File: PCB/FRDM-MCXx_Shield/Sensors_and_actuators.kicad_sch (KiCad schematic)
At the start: 15 parts, among them M1 Motor_Servo, U2 M95010-RMN6TP, U3 LM35-D

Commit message: Fixed labeling
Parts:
- U2: footprint SOIC127P600X175-8N -> SamacSys:SOIC127P600X175-8N
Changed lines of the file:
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@@
 			)
 		)
-		(property "Footprint" "SOIC127P600X175-8N"
+		(property "Footprint" "SamacSys:SOIC127P600X175-8N"
 			(at 251.46 213.03 0)
 			(effects

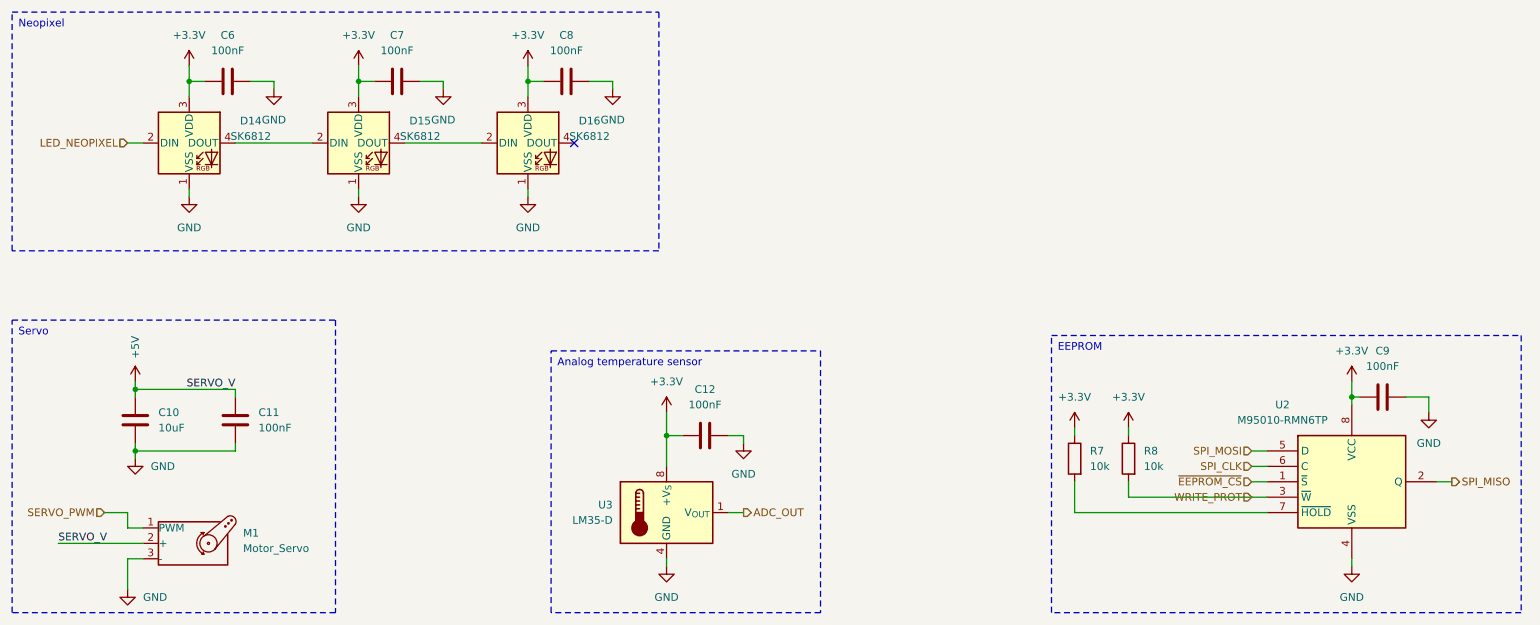
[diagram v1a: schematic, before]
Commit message: Updated PCB
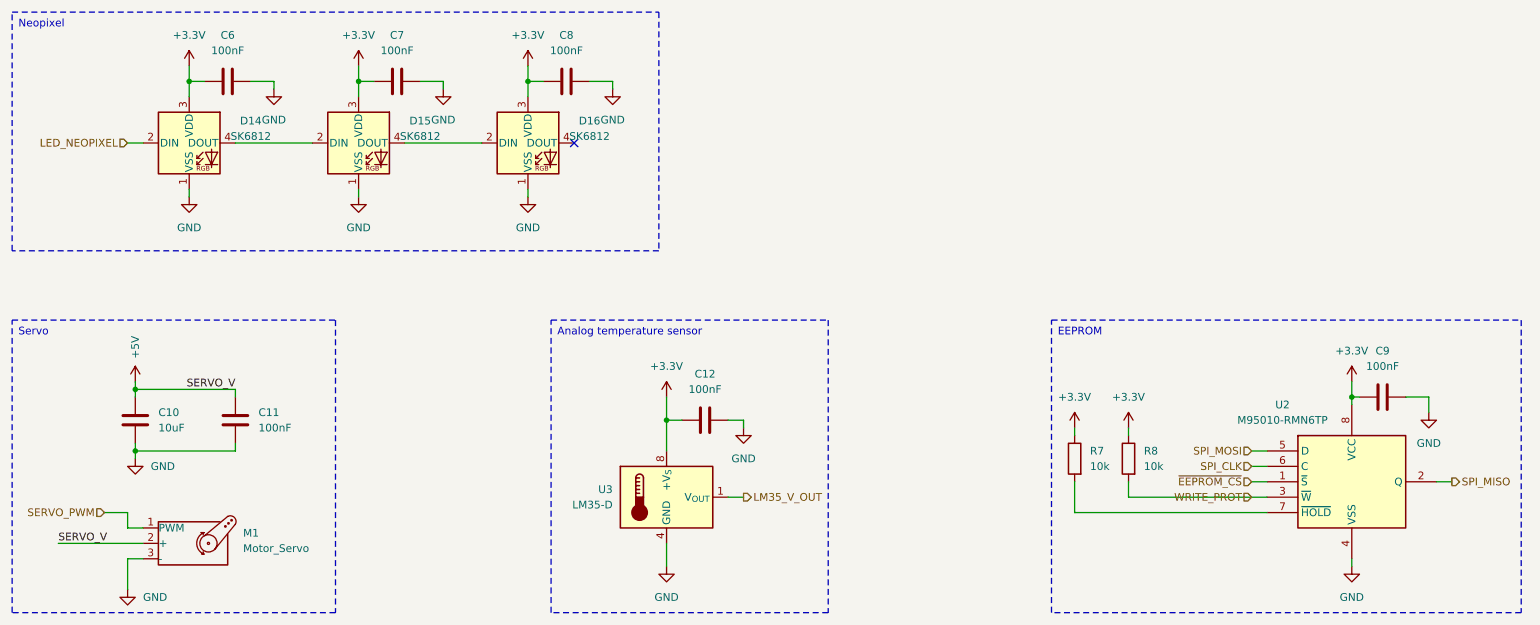
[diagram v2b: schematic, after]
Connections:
- net ADC_OUT renamed LM35_V_OUT
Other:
- moved on the sheet: C12, U3
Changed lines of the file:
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@@
 	(title_block
 		(title "Sensors & actuators")
-		(date "2024-04-26")
+		(date "2024-05-05")
 		(rev "V2.0")
 		(company "HAN")
@@
 	)
 	(junction
-		(at 128.27 113.03)
+		(at 128.27 110.49)
 		(diameter 0)
 		(color 0 0 0 0)
@@
 	(wire
 		(pts
-			(xy 128.27 133.35) (xy 128.27 134.62)
+			(xy 128.27 130.81) (xy 128.27 134.62)
 		)
 		(stroke
@@
 	(wire
 		(pts
-			(xy 130.81 113.03) (xy 128.27 113.03)
-		)
-		(stroke
-			(width 0)
-			(type default)
-		)
-	)
-	(wire
-		(pts
-			(xy 140.97 113.03) (xy 138.43 113.03)
+			(xy 130.81 110.49) (xy 128.27 110.49)
+		)
+		(stroke
+			(width 0)
+			(type default)
+		)
+	)
+	(wire
+		(pts
+			(xy 140.97 110.49) (xy 138.43 110.49)
 		)
 		(stroke
@@
 	(wire
 		(pts
-			(xy 128.27 109.22) (xy 128.27 113.03)
+			(xy 128.27 106.68) (xy 128.27 110.49)
 		)
 		(stroke
@@
 	(wire
 		(pts
-			(xy 140.97 114.3) (xy 140.97 113.03)
+			(xy 140.97 111.76) (xy 140.97 110.49)
 		)
 		(stroke
@@
 	(wire
 		(pts
-			(xy 138.43 125.73) (xy 140.97 125.73)
+			(xy 138.43 123.19) (xy 140.97 123.19)
 		)
 		(stroke
@@
 	(wire
 		(pts
-			(xy 128.27 113.03) (xy 128.27 118.11)
+			(xy 128.27 110.49) (xy 128.27 115.57)
 		)
 		(stroke
@@
 	(text_box "Analog temperature sensor"
 		(exclude_from_sim no)
-		(at 109.22 99.06 0)
-		(size 44.45 43.18)
+		(at 109.22 93.98 0)
+		(size 45.72 48.26)
 		(stroke
 			(width 0)
@@
 	(text_box "EEPROM"
 		(exclude_from_sim no)
-		(at 191.77 96.52 0)
-		(size 77.47 45.72)
+		(at 191.77 93.98 0)
+		(size 77.47 48.26)
 		(stroke
 			(width 0)
@@
 		)
 	)
-	(hierarchical_label "ADC_OUT"
+	(hierarchical_label "LM35_V_OUT"
 		(shape output)
-		(at 140.97 125.73 0)
+		(at 140.97 123.19 0)
 		(fields_autoplaced yes)
 		(effects
@@
 	(symbol
 		(lib_id "Device:C")
-		(at 134.62 113.03 90)
+		(at 134.62 110.49 90)
 		(unit 1)
 		(exclude_from_sim no)
@@
 		(fields_autoplaced yes)
 		(property "Reference" "C12"
+			(at 134.62 102.87 90)
+			(effects
+				(font
+					(size 1.27 1.27)
+				)
+			)
+		)
+		(property "Value" "100nF"
 			(at 134.62 105.41 90)
 			(effects
@@
 			)
 		)
-		(property "Value" "100nF"
-			(at 134.62 107.95 90)
-			(effects
-				(font
-					(size 1.27 1.27)
-				)
-			)
-		)
 		(property "Footprint" "Capacitor_SMD:C_0805_2012Metric_Pad1.18x1.45mm_HandSolder"
-			(at 138.43 112.0648 0)
+			(at 138.43 109.5248 0)
 			(effects
 				(font
@@
 		)
 		(property "Datasheet" "~"
-			(at 134.62 113.03 0)
+			(at 134.62 110.49 0)
 			(effects
 				(font
@@
 		)
 		(property "Description" ""
-			(at 134.62 113.03 0)
+			(at 134.62 110.49 0)
 			(effects
 				(font
@@
 		)
 		(property "GPN" "GPC0603104"
-			(at 134.62 113.03 90)
+			(at 134.62 110.49 90)
 			(effects
 				(font
@@
 	(symbol
 		(lib_id "power:+3.3V")
-		(at 128.27 109.22 0)
+		(at 128.27 106.68 0)
 		(unit 1)
 		(exclude_from_sim no)
@@
 		(fields_autoplaced yes)
 		(property "Reference" "#PWR044"
-			(at 128.27 113.03 0)
+			(at 128.27 110.49 0)
 			(effects
 				(font
@@
 		)
 		(property "Value" "+3.3V"
-			(at 128.27 104.14 0)
+			(at 128.27 101.6 0)
 			(effects
 				(font
@@
 		)
 		(property "Footprint" ""
-			(at 128.27 109.22 0)
+			(at 128.27 106.68 0)
 			(effects
 				(font
@@
 		)
 		(property "Datasheet" ""
-			(at 128.27 109.22 0)
+			(at 128.27 106.68 0)
 			(effects
 				(font
@@
 		)
 		(property "Description" ""
-			(at 128.27 109.22 0)
+			(at 128.27 106.68 0)
 			(effects
 				(font
@@
 	(symbol
 		(lib_id "power:GND")
-		(at 140.97 114.3 0)
+		(at 140.97 111.76 0)
 		(unit 1)
 		(exclude_from_sim no)
@@
 		(fields_autoplaced yes)
 		(property "Reference" "#PWR048"
-			(at 140.97 120.65 0)
+			(at 140.97 118.11 0)
 			(effects
 				(font
@@
 		)
 		(property "Value" "GND"
-			(at 140.97 119.38 0)
+			(at 140.97 116.84 0)
 			(effects
 				(font
@@
 		)
 		(property "Footprint" ""
-			(at 140.97 114.3 0)
+			(at 140.97 111.76 0)
 			(effects
 				(font
@@
 		)
 		(property "Datasheet" ""
-			(at 140.97 114.3 0)
+			(at 140.97 111.76 0)
 			(effects
 				(font
@@
 		)
 		(property "Description" ""
-			(at 140.97 114.3 0)
+			(at 140.97 111.76 0)
 			(effects
 				(font
@@
 	(symbol
 		(lib_id "Sensor_Temperature:LM35-D")
-		(at 128.27 125.73 0)
+		(at 128.27 123.19 0)
 		(unit 1)
 		(exclude_from_sim no)
@@
 		(fields_autoplaced yes)
 		(property "Reference" "U3"
+			(at 119.38 121.9199 0)
+			(effects
+				(font
+					(size 1.27 1.27)
+				)
+				(justify right)
+			)
+		)
+		(property "Value" "LM35-D"
 			(at 119.38 124.4599 0)
 			(effects
@@
 			)
 		)
-		(property "Value" "LM35-D"
-			(at 119.38 126.9999 0)
-			(effects
-				(font
-					(size 1.27 1.27)
-				)
-				(justify right)
-			)
-		)
 		(property "Footprint" "Package_SO:SOIC-8_3.9x4.9mm_P1.27mm"
-			(at 128.27 135.89 0)
+			(at 128.27 133.35 0)
 			(effects
 				(font
@@
 		)
 		(property "Datasheet" "http://www.ti.com/lit/ds/symlink/lm35.pdf"
-			(at 128.27 125.73 0)
+			(at 128.27 123.19 0)
 			(effects
 				(font
@@
 		)
 		(property "Description" "Precision centigrade temperature sensor, SOIC-8"
-			(at 128.27 125.73 0)
-			(effects
-				(font
+			(at 128.27 123.19 0)
+			(effects
+				(font
